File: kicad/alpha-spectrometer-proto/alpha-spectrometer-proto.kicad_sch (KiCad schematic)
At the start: 78 parts, among them J1 USB_B_Micro, J13 Anode, J14 Catode, J19 Conn, J2 Conn_01x01_Female, J20 Conn_01x01_Female, J21 Conn_01x01_Female, J22 Conn_01x01_Female, J3 Conn_01x01_Female, J4 BAT+, J5 BAT-, Q1 IRLML5203, SW1 SW_Push_SPDT, U1 MAX4477, U2 LM2733XMF, U3 MCP73831, U5 LMV7239, U6 MCP1700x, U7 LT3045xMSE, Y1 16

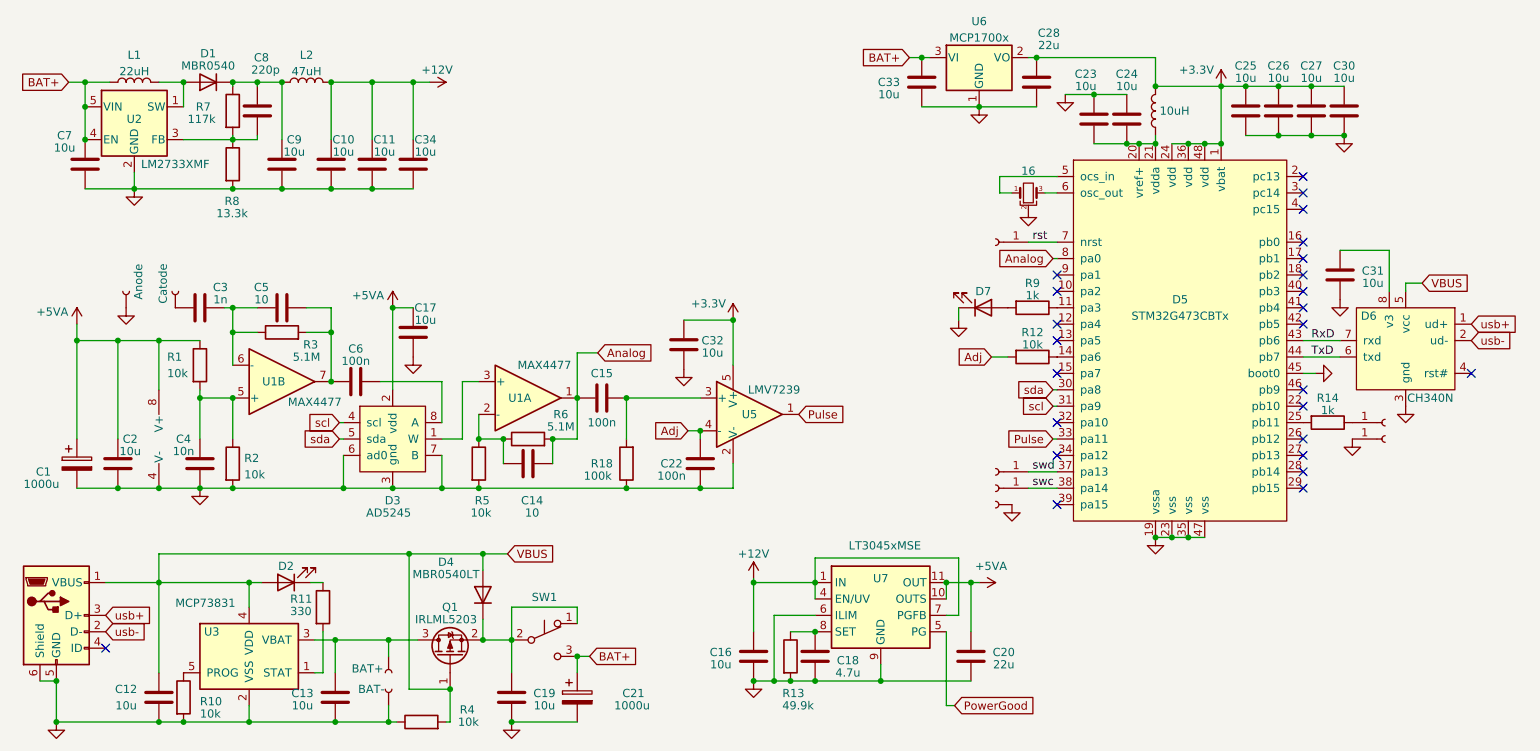
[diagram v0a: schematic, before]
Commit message: удалено:       Documents/mr107+-1.png 	удалено:       Documents/mr107+-10.png 	удалено:       Documents/mr107+-11.png 	удалено:       Documents/mr107+-12.png 	удалено:       Documents/mr107+-13.png 	удалено:       Documents/mr107+-14.png 	удалено:       Documents/mr107+-2.png 	удалено:       Documents/mr107+-3.png 	удалено:       Documents/mr107+-4.png 	удалено:       Documents/mr107+-5.png 	удалено:       Documents/mr107+-6.png 	удалено:       Documents/mr107+-7.png 	удалено:       Documents/mr107+-8.png 	удалено:       Documents/mr107+-9.png 	изменено:      GNUPlot/mainChart-1.gp 	изменено:      GNUPlot/mainChart-1.gp~ 	изменено:      STM32CubeIDE/TestController/.settings/language.settings.xml 	изменено:      STM32CubeIDE/TestController/Core/Src/main.c 	изменено:      STM32CubeIDE/TestController/Debug/Core/Src/main.o 	изменено:      STM32CubeIDE/TestController/Debug/TestController.elf 	изменено:      STM32CubeIDE/TestController/Debug/TestController.list 	изменено:      STM32CubeIDE/TestController/TestController.ioc 	удалено:       kicad/alpha-spectrometer-proto/alpha-spectrometer-proto-backups/alpha-spectrometer-proto-2024-10-29_185625.zip 	удалено:       kicad/alpha-spectrometer-proto/alpha-spectrometer-proto-backups/alpha-spectrometer-proto-2024-10-29_190534.zip 	удалено:       kicad/alpha-spectrometer-proto/alpha-spectrometer-proto-backups/alpha-spectrometer-proto-2024-10-30_170209.zip 	удалено:       kicad/alpha-spectrometer-proto/alpha-spectrometer-proto-backups/alpha-spectrometer-proto-2024-10-30_171711.zip 	удалено:       kicad/alpha-spectrometer-proto/alpha-spectrometer-proto-backups/alpha-spectrometer-proto-2024-10-30_184706.zip 	удалено:       kicad/alpha-spectrometer-proto/alpha-spectrometer-proto-backups/alpha-spectrometer-proto-2024-10-30_185305.zip 	удалено:       kicad/alpha-spectrometer-proto/alpha-spectrometer-proto-backups/alpha-spectrometer-proto-2024-10-30_190038.zip 	удалено:       kicad/alpha-spectrometer-proto/alpha-spectrometer-proto-backup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
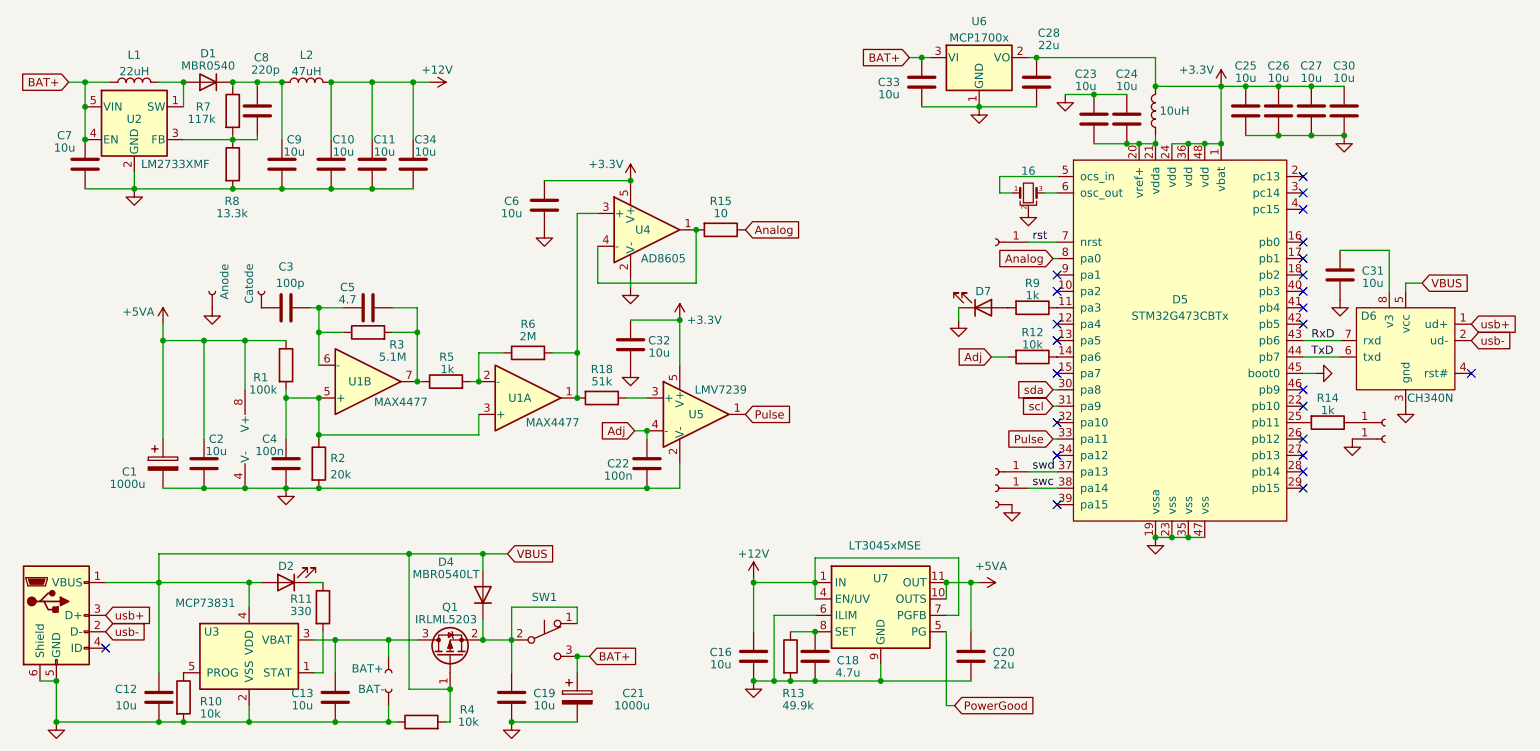
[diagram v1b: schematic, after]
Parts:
- removed C14: 10, Capacitor_SMD:C_0603_1608Metric, symbol Device:C
- removed C15: 100n, Capacitor_SMD:C_0603_1608Metric, symbol Device:C
- removed C17: 10u, Capacitor_SMD:C_0603_1608Metric, symbol Device:C
- removed D3: AD5245, Package_TO_SOT_SMD:SOT-23-8_Handsoldering, symbol Anemometer_200_G473-rescue:AD5245-My_Library-My_Library-Anemometer_200_G473-res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
- added R15: 10, Resistor_SMD:R_0603_1608Metric, symbol Device:R
- added U4: AD8605, Package_TO_SOT_SMD:TSOT-23-5, symbol Amplifier_Operational:AD8603
- C3: value 1n -> 100p
- C4: value 10n -> 100n
- C5: value 10 -> 4.7
- C6: value 100n -> 10u
- R1: value 10k -> 100k
- R18: value 100k -> 51k
- R2: value 10k -> 20k
- R5: value 10k -> 1k
- R6: value 5.1M -> 2M
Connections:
- net +3V3: now also C6.2, U4.5 (V+)
- net Analog: now also R15.1; no longer R6.2, U1.1
- net GND: now also C6.1, U4.2 (V-); no longer R18.1, R5.2
- net at R6.1, U1.2 (-): now also R5.2; no longer R5.1
- net at U1.3 (+): now also C4.2, R1.2, R2.1, U1.5 (+)
- net at C5.2, R3.2, U1.7: now also R5.1; no longer C6.1
- net at R18.2: now also R6.2, U1.1, U4.3 (+); no longer U5.3 (+)
- new net: R15.2, U4.1, U4.4 (-)
- new net: R18.1, U5.3 (+)
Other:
- moved on the sheet: C1, C2, C22, C3, C32, C4, C5, R1, R18, R2, R3, R5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
